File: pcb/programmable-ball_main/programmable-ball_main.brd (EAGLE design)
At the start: 30 x 30 mm, 30 parts, among them J1 12402012E212A, J3 B4B-ZR-SM4-TFT(LF)(SN), P1 S2B-ZR-SM4A-TF, Q1 DMG2305UX-13, U1 MDBT50Q-1MV2, U2 AP2112K-3.3TRG1, U3 MCP73832T-2ACI/OT, Y1 FC-135_32.7680KA-A0

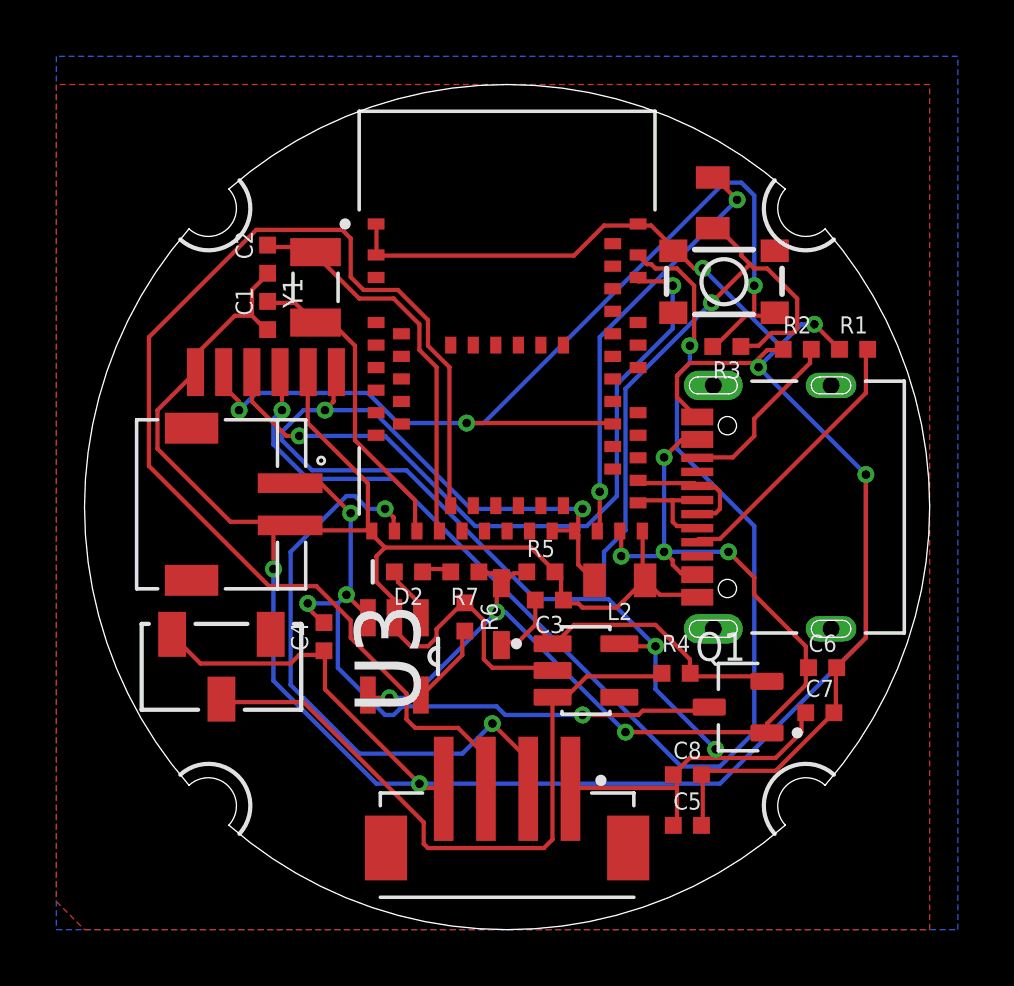
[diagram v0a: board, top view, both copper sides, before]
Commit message: v1の修正
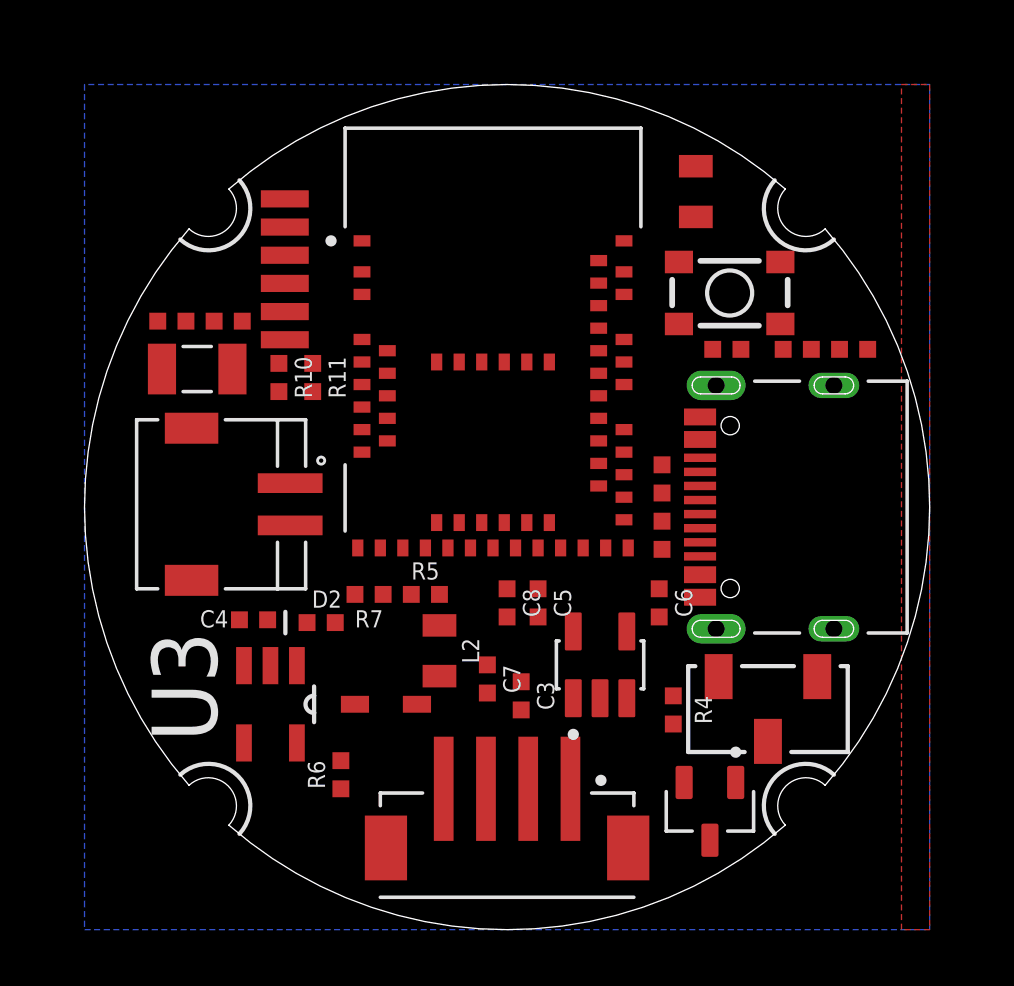
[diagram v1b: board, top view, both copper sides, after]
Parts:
- added R10, R11: 100k, SparkFun-Resistors:0402-TIGHT
- added R8, R9: 22Ω, SparkFun-Resistors:0402-TIGHT
- moved S2 19.5 mm to (26.8, 9.10)
- moved C7 11.9 mm to (14.3, 8.90), turned to 270 degrees
- moved C5 9.51 mm to (16.1, 11.6), turned to 270 degrees
- moved C8 8.84 mm to (15.0, 11.6), turned to 270 degrees
- moved R6 7.12 mm to (9.10, 5.50), turned to 90 degrees
- moved L2 6.87 mm to (12.6, 9.90), turned to 90 degrees
- moved C6 6.24 mm to (20.4, 11.6), turned to 270 degrees
- moved D1 5.20 mm to (10.7, 8.00), turned to 180 degrees
- moved Y1 5.10 mm to (4.00, 19.9), turned to 0 degrees
- moved U3 4.72 mm to (6.60, 8.00)
- moved R5 4.18 mm to (12.1, 11.9)
- moved Q1 3.83 mm to (22.2, 4.20), turned to 270 degrees
- moved D2 3.58 mm to (8.40, 10.9)
- moved C3 3.54 mm to (15.5, 8.30), turned to 270 degrees
- moved R7 3.49 mm to (10.1, 11.9)
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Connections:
- new net N$10: R8.1, U1.35
- new net N$11: R9.1, U1.34
- new net VDIV: R10.1, R11.2, U1.10
- net GND: now also R11.1
- net USBD+: now also R8.2; no longer U1.35
- net USBD-: now also R9.2; no longer U1.34
- net VBAT: now also R10.2
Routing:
- net GND: track 151.1 -> 0.00 mm, vias 6 -> 0
- net 3.3V: track 73.8 -> 0.00 mm, vias 5 -> 0
- net SWDCLK: track 44.7 -> 0.00 mm, vias 2 -> 0
- net I2C_SDA: track 43.4 -> 0.00 mm
- net VBUS: track 39.8 -> 0.00 mm, vias 7 -> 0
- net RESET: track 36.4 -> 0.00 mm, vias 3 -> 0
- net SWDIO: track 26.0 -> 0.00 mm, vias 2 -> 0
- net VBAT: track 25.7 -> 0.00 mm, vias 4 -> 0
- net EN: track 23.9 -> 0.00 mm
- net I2C_SCL: track 21.5 -> 0.00 mm, vias 2 -> 0
- net N$5: track 15.0 -> 0.00 mm, vias 2 -> 0
- net N$3: track 14.3 -> 0.00 mm
- net N$6: track 12.3 -> 0.00 mm
- net N$4: track 11.3 -> 0.00 mm
- net N$1: track 9.81 -> 0.00 mm
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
